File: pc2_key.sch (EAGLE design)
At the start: 52 parts, among them J2 0

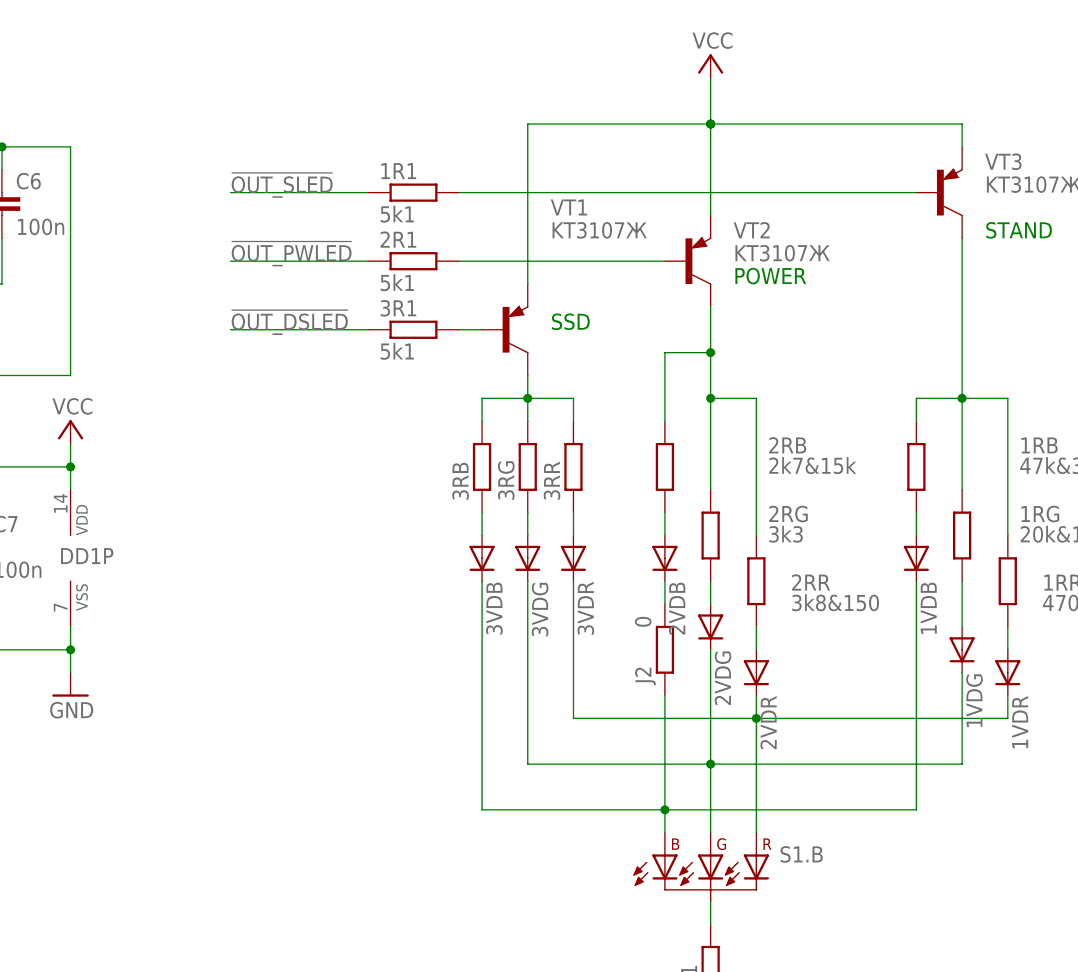
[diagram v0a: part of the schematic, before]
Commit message: .
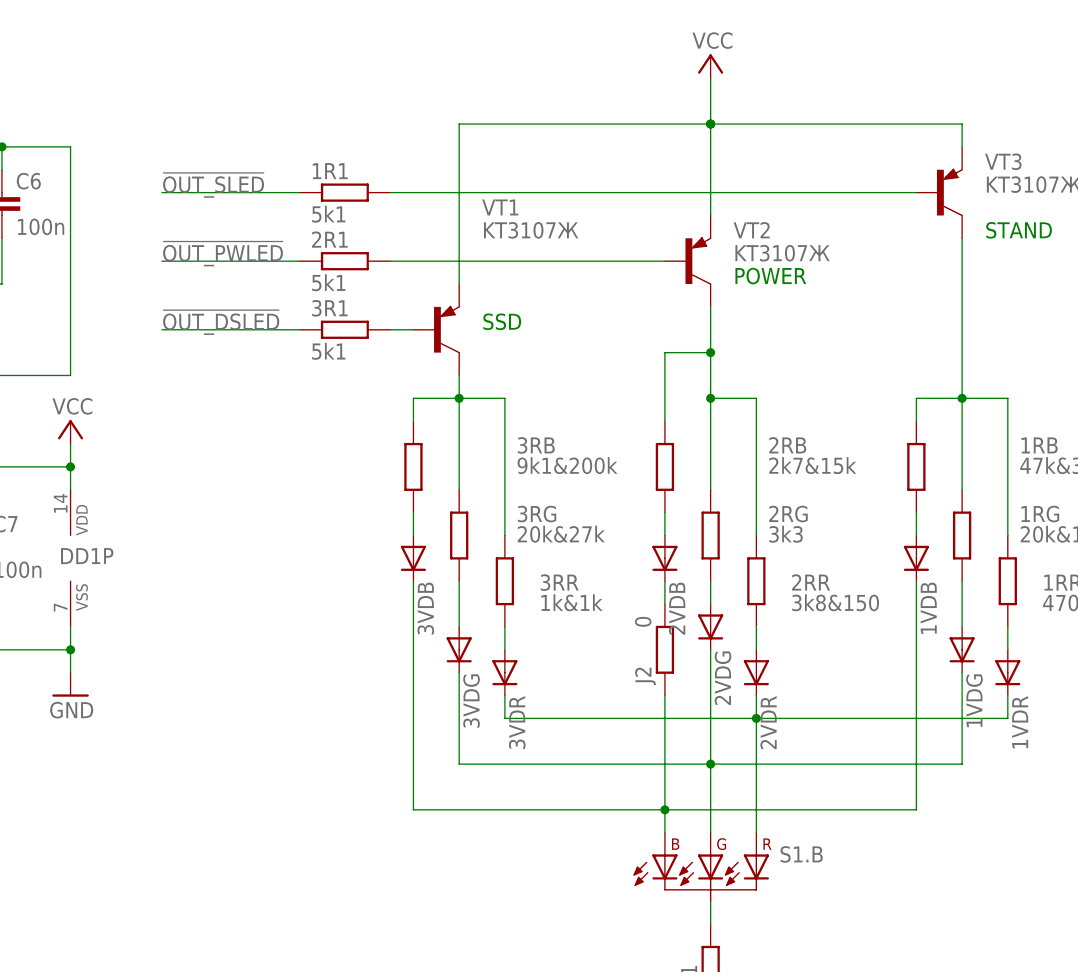
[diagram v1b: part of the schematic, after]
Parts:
- 3RB: value (none) -> 9k1&200k
- 3RG: value (none) -> 20k&27k
- 3RR: value (none) -> 1k&1k
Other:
- moved on the sheet: 1R1, 2R1, 3R1, 3RB, 3RG, 3RR, 3VDB, 3VDG, 3VDR, VT1
